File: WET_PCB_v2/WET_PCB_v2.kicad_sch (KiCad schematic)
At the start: 41 parts, among them J10 Conn_01x09_Pin, J11 Conn_01x09_Pin, J16 POGO1, J2 Conn_01x09_Pin, J21 POGO2, J26 Vsense_ADC1_IN1, J3 Conn_01x09_Pin, J4 Power input, J5 Barrel jack, J6 Coil plug, J7 Pluggable Terminal Block, J8 Jumper, U3 Opamp_Quad

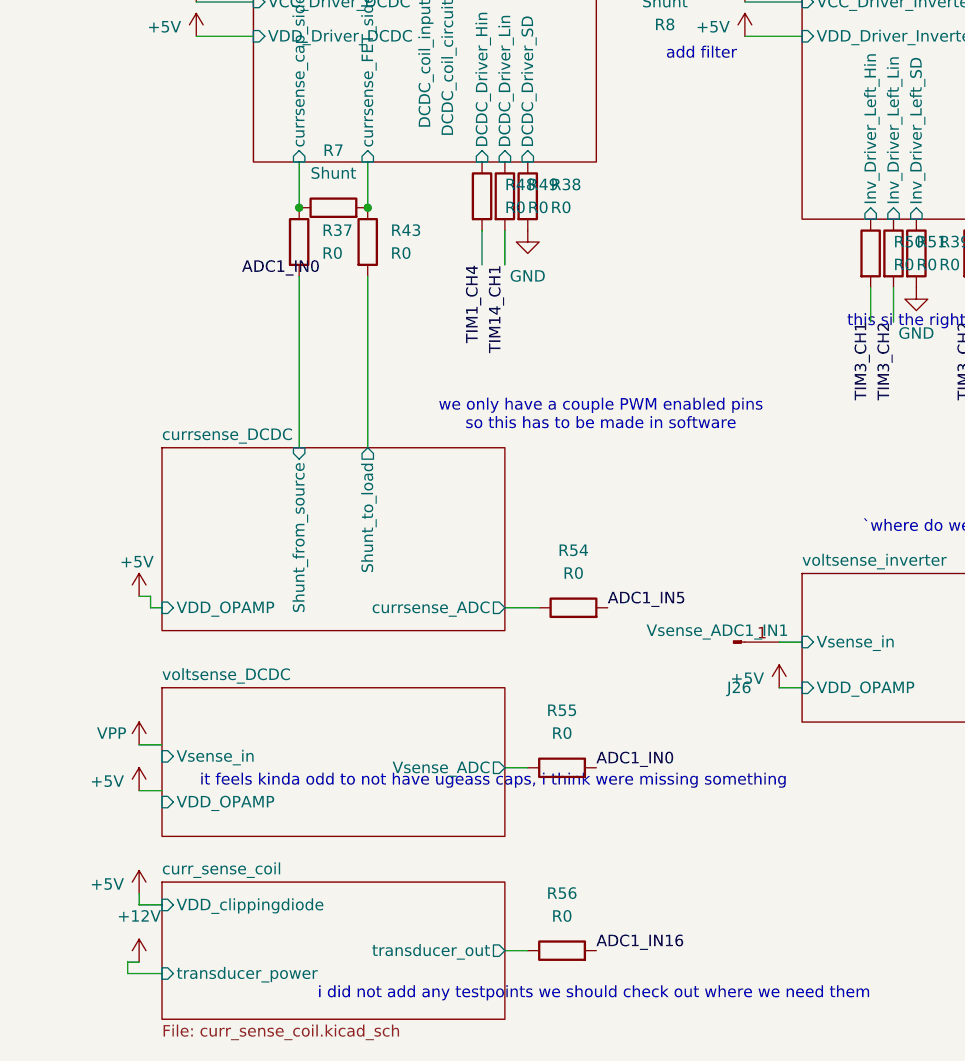
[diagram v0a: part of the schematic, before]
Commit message: veel routes weinig goeds
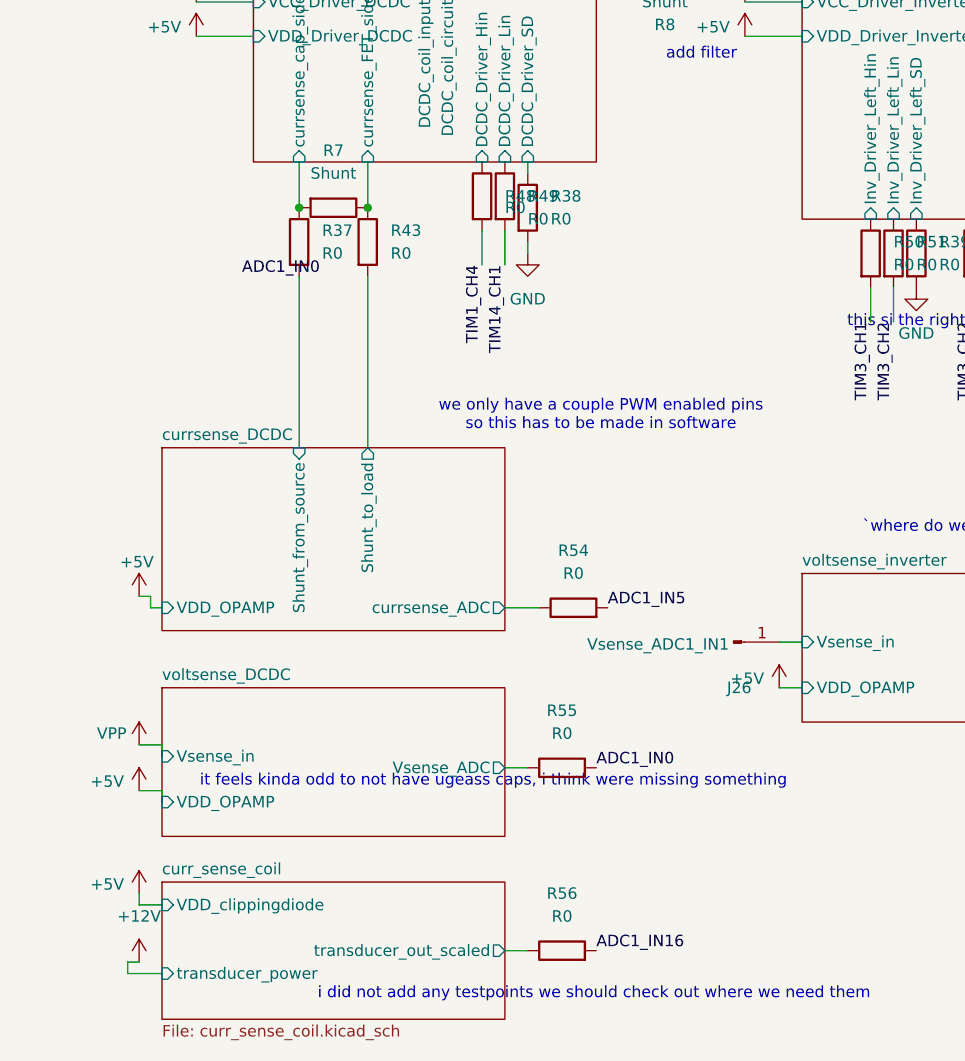
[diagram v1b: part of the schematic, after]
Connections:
- net DCDC/currsense_FET_side: now also R7.1; no longer R7.2
- net DCDC/currsense_cap_side: now also R7.2; no longer R7.1
- net curr_sense_coil/transducer_out renamed curr_sense_coil/transducer_out_scaled
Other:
- sheet curr_sense_coil ports: added transducer_out_scaled; removed transducer_out
- moved on the sheet: R38, R7
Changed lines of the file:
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@@
 	)
 	(junction
+		(at 149.86 85.09)
+		(diameter 0)
+		(color 0 0 0 0)
+	)
+	(junction
 		(at 194.31 58.42)
 		(diameter 0)
@@
 		(color 0 0 0 0)
 	)
-	(junction
-		(at 149.86 85.09)
-		(diameter 0)
-		(color 0 0 0 0)
-	)
 	(wire
 		(pts
@@
 	(wire
 		(pts
+			(xy 134.62 144.78) (xy 134.62 146.05)
+		)
+		(stroke
+			(width 0)
+			(type default)
+		)
+	)
+	(wire
+		(pts
 			(xy 53.34 77.47) (xy 69.85 77.47)
 		)
@@
 	(wire
 		(pts
+			(xy 175.26 81.28) (xy 175.26 80.01)
+		)
+		(stroke
+			(width 0)
+			(type default)
+		)
+	)
+	(wire
+		(pts
 			(xy 29.21 114.3) (xy 26.67 114.3)
 		)
@@
 	(wire
 		(pts
+			(xy 134.62 149.86) (xy 134.62 151.13)
+		)
+		(stroke
+			(width 0)
+			(type default)
+		)
+	)
+	(wire
+		(pts
 			(xy 373.38 152.4) (xy 387.35 152.4)
 		)
@@
 	(wire
 		(pts
+			(xy 175.26 90.17) (xy 175.26 88.9)
+		)
+		(stroke
+			(width 0)
+			(type default)
+		)
+	)
+	(wire
+		(pts
 			(xy 69.85 77.47) (xy 86.36 77.47)
 		)
@@
 	(symbol
 		(lib_id "Device:R")
-		(at 153.67 85.09 90)
+		(at 153.67 85.09 270)
 		(unit 1)
 		(body_style 1)
@@
 		)
 		(property "Footprint" "Resistor_SMD:R_2512_6332Metric_Pad1.40x3.35mm_HandSolder"
-			(at 153.67 86.868 90)
+			(at 153.67 83.312 90)
 			(hide yes)
 			(show_name no)
@@
 		)
 		(property "Value" "Vsense_ADC1_IN1"
-			(at 196.342 132.08 0)
+			(at 189.738 133.604 0)
 			(show_name no)
 			(do_not_autoplace no)
@@
 	(symbol
 		(lib_id "Device:R")
-		(at 175.26 83.82 0)
+		(at 175.26 85.09 0)
 		(unit 1)
 		(body_style 1)
@@
 		(fields_autoplaced yes)
 		(property "Reference" "R38"
-			(at 177.8 82.5499 0)
+			(at 177.8 83.8199 0)
 			(show_name no)
 			(do_not_autoplace no)
@@
 		)
 		(property "Value" "R0"
-			(at 177.8 85.0899 0)
+			(at 177.8 86.3599 0)
 			(show_name no)
 			(do_not_autoplace no)
@@
 		)
 		(property "Footprint" "Resistor_SMD:R_0805_2012Metric_Pad1.20x1.40mm_HandSolder"
-			(at 173.482 83.82 90)
+			(at 173.482 85.09 90)
 			(hide yes)
 			(show_name no)
@@
 		)
 		(property "Datasheet" ""
-			(at 175.26 83.82 0)
+			(at 175.26 85.09 0)
 			(hide yes)
 			(show_name no)
@@
 		)
 		(property "Description" "Resistor"
-			(at 175.26 83.82 0)
+			(at 175.26 85.09 0)
 			(hide yes)
 			(show_name no)
@@
 	(symbol
 		(lib_id "power:GND")
-		(at 175.26 87.63 0)
+		(at 175.26 90.17 0)
 		(unit 1)
 		(body_style 1)
@@
 		(fields_autoplaced yes)
 		(property "Reference" "#PWR051"
-			(at 175.26 93.98 0)
+			(at 175.26 96.52 0)
 			(hide yes)
 			(show_name no)
@@
 		)
 		(property "Value" "GND"
-			(at 175.26 92.71 0)
+			(at 175.26 95.25 0)
 			(show_name no)
 			(do_not_autoplace no)
@@
 		)
 		(property "Footprint" ""
-			(at 175.26 87.63 0)
+			(at 175.26 90.17 0)
 			(hide yes)
 			(show_name no)
@@
 		)
 		(property "Datasheet" ""
-			(at 175.26 87.63 0)
+			(at 175.26 90.17 0)
 			(hide yes)
 			(show_name no)
@@
 		)
 		(property "Description" "Power symbol creates a global label with name \"GND\" , ground"
-			(at 175.26 87.63 0)
+			(at 175.26 90.17 0)
 			(hide yes)
 			(show_name no)
@@
 		(in_pos_files yes)
 		(dnp no)
-		(fields_autoplaced yes)
 		(property "Reference" "R49"
-			(at 175.26 82.5499 0)
+			(at 175.26 83.8199 0)
 			(show_name no)
 			(do_not_autoplace no)
@@
 		)
 		(property "Value" "R0"
-			(at 175.26 85.0899 0)
+			(at 175.26 86.3599 0)
 			(show_name no)
 			(do_not_autoplace no)
@@
 		(in_pos_files yes)
 		(dnp no)
-		(fields_autoplaced yes)
 		(property "Reference" "R48"
-			(at 172.72 82.5499 0)
+			(at 172.72 83.8199 0)
 			(show_name no)
 			(do_not_autoplace no)
@@
 			)
 		)
-		(pin "transducer_out" output
+		(pin "transducer_out_scaled" output
 			(at 172.72 167.64 0)
 			(effects
